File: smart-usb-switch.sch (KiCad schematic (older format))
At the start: 8 parts, among them J1 USB_A, J2 USB_A, J3 Conn_01x04, J4 Conn_01x02, Q1 2N7002E, U1 ESP-12F, U2 TLV75533PDBV

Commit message: more docs, updates
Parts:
- U2: symbol Regulator_Linear:TLV75533PDBV -> smart-usb-switch-rescue:TLV75533PDBV-Regulator_Linear
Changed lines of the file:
@@
 EESchema Schematic File Version 4
-EELAYER 26 0
+EELAYER 30 0
 EELAYER END
 $Descr A4 11693 8268
@@
 	5700 2100 5700 2400
 $Comp
-L Regulator_Linear:TLV75533PDBV U2
+L smart-usb-switch-rescue:TLV75533PDBV-Regulator_Linear U2
 U 1 1 5DE30043
 P 4250 2900

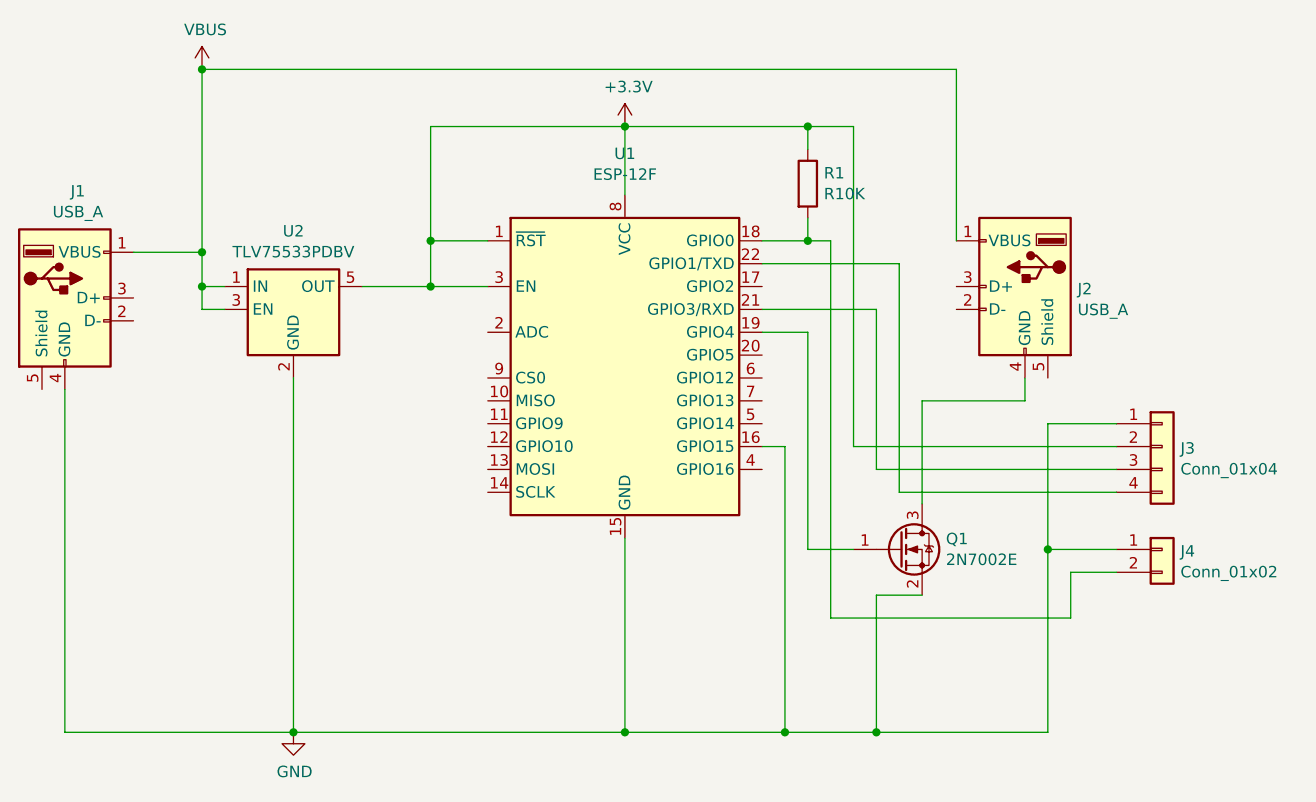
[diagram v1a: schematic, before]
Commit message: reroute
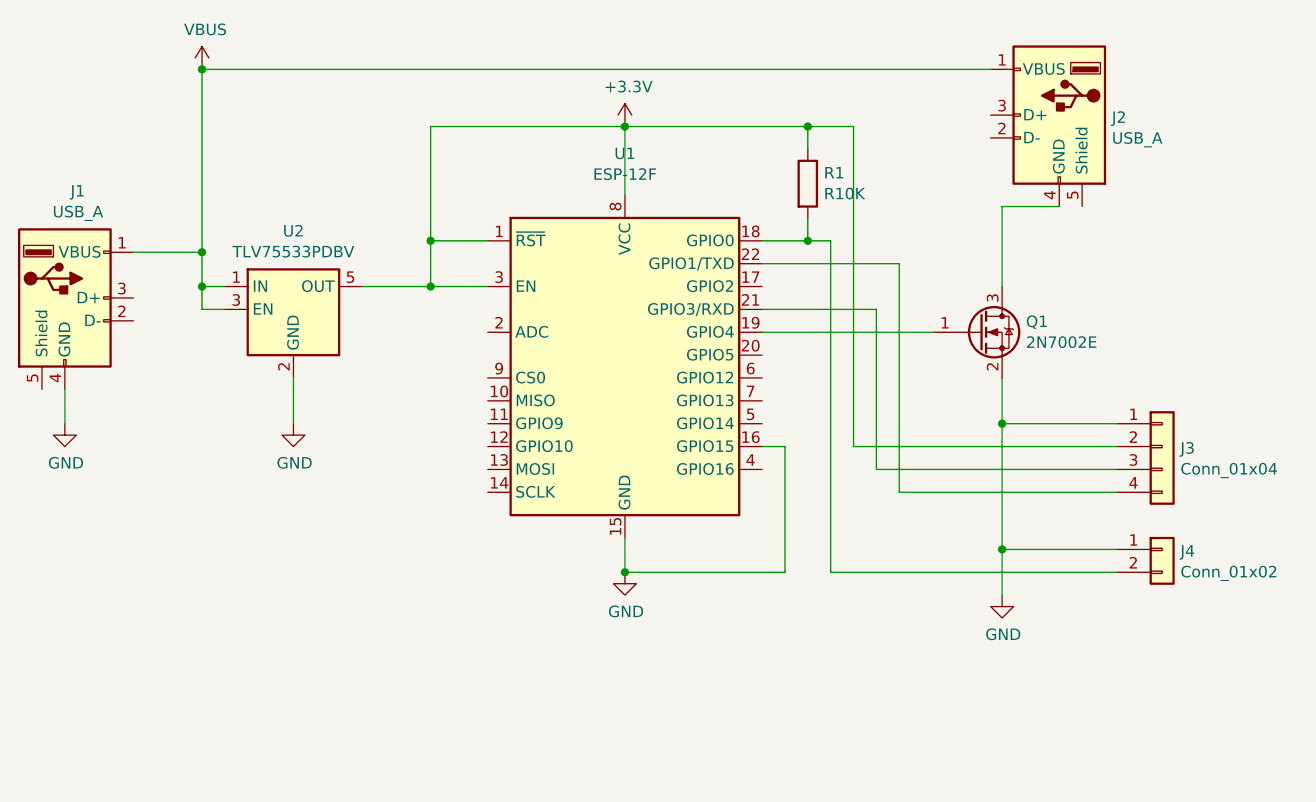
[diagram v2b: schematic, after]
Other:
- moved on the sheet: J2, Q1
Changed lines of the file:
@@
 $EndComp
 Wire Wire Line
-	3250 4750 4250 4750
-Wire Wire Line
-	5700 4750 5700 3900
+	5700 4050 5700 3900
 Wire Wire Line
 	3550 2650 3850 2650
@@
 L Connector:USB_A J2
 U 1 1 5DE34A4B
-P 7450 2800
-F 0 "J2" H 7220 2789 50  0000 R CNN
-F 1 "USB_A" H 7220 2698 50  0000 R CNN
-F 2 "Connector_USB:USB_A_Stewart_SS-52100-001_Horizontal" H 7600 2750 50  0001 C CNN
-F 3 " ~" H 7600 2750 50  0001 C CNN
-	1    7450 2800
+P 7600 2050
+F 0 "J2" H 7370 2039 50  0000 R CNN
+F 1 "USB_A" H 7370 1948 50  0000 R CNN
+F 2 "Connector_USB:USB_A_Stewart_SS-52100-001_Horizontal" H 7750 2000 50  0001 C CNN
+F 3 " ~" H 7750 2000 50  0001 C CNN
+	1    7600 2050
 	-1   0    0    -1
 $EndComp
-Wire Wire Line
-	7450 3200 7450 3300
-Connection ~ 5700 4750
-Wire Wire Line
-	6800 4150 6800 4750
-Connection ~ 6800 4750
-Wire Wire Line
-	6800 4750 6400 4750
-Wire Wire Line
-	6800 4750 7550 4750
+Connection ~ 5700 4050
 $Comp
 L power:GND #PWR0101
 U 1 1 5DE35A33
-P 4250 4750
-F 0 "#PWR0101" H 4250 4500 50  0001 C CNN
-F 1 "GND" H 4255 4577 50  0000 C CNN
-F 2 "" H 4250 4750 50  0001 C CNN
-F 3 "" H 4250 4750 50  0001 C CNN
-	1    4250 4750
+P 4250 3400
+F 0 "#PWR0101" H 4250 3150 50  0001 C CNN
+F 1 "GND" H 4255 3227 50  0000 C CNN
+F 2 "" H 4250 3400 50  0001 C CNN
+F 3 "" H 4250 3400 50  0001 C CNN
+	1    4250 3400
 	1    0    0    -1
 $EndComp
@@
 Connection ~ 5700 2100
 Wire Wire Line
-	7150 2600 7150 1850
-Wire Wire Line
-	7150 1850 3850 1850
-Wire Wire Line
 	3850 1850 3850 2650
 Connection ~ 3850 2650
-Wire Wire Line
-	6800 4150 7000 4150
 $Comp
 L Connector_Generic:Conn_01x04 J3
@@
 	6700 2100 6500 2100
 Wire Wire Line
-	7850 3400 7550 3400
-Wire Wire Line
-	7550 3400 7550 3950
-Wire Wire Line
 	6800 2900 6800 3600
 $Comp
@@
 	6300 2600 6500 2600
 Wire Wire Line
-	6600 2600 6600 4250
-Wire Wire Line
-	7850 4050 7650 4050
-Wire Wire Line
-	6700 3950 6500 3950
-Wire Wire Line
-	6600 4250 7650 4250
-Wire Wire Line
-	7650 4250 7650 4050
-Wire Wire Line
-	7550 3950 7850 3950
-Connection ~ 7550 3950
-Wire Wire Line
-	7550 3950 7550 4750
-Wire Wire Line
-	4250 3200 4250 4750
-Connection ~ 4250 4750
+	6600 2600 6600 4050
+Wire Wire Line
+	7350 3950 7850 3950
+Wire Wire Line
+	4250 3200 4250 3400
 $Comp
 L Transistor_FET:2N7002E Q1
 U 1 1 5DE386B7
-P 6900 3950
-F 0 "Q1" H 7104 3996 50  0000 L CNN
-F 1 "2N7002E" H 7104 3905 50  0000 L CNN
-F 2 "Package_TO_SOT_SMD:SOT-23" H 7100 3875 50  0001 L CIN
-F 3 "http://www.diodes.com/assets/Datasheets/ds30376.pdf" H 6900 3950 50  0001 L CNN
-	1    6900 3950
+P 7250 3000
+F 0 "Q1" H 7454 3046 50  0000 L CNN
+F 1 "2N7002E" H 7454 2955 50  0000 L CNN
+F 2 "Package_TO_SOT_SMD:SOT-23" H 7450 2925 50  0001 L CIN
+F 3 "http://www.diodes.com/assets/Datasheets/ds30376.pdf" H 7250 3000 50  0001 L CNN
+	1    7250 3000
 	1    0    0    -1
 $EndComp
@@
 	6300 3500 6400 3500
 Wire Wire Line
-	6400 3500 6400 4750
-Connection ~ 6400 4750
-Wire Wire Line
-	6400 4750 5700 4750
+	6400 3500 6400 4050
+Wire Wire Line
+	6400 4050 5700 4050
 $Comp
 L Device:R R1
@@
 Connection ~ 3850 1850
 Wire Wire Line
-	4250 4750 5700 4750
-Wire Wire Line
-	3250 3250 3250 4750
-Wire Wire Line
-	7000 3750 7000 3300
-Wire Wire Line
-	7000 3300 7450 3300
-Wire Wire Line
-	6500 3000 6300 3000
-Wire Wire Line
-	6500 3000 6500 3950
+	3250 3250 3250 3400
+Wire Wire Line
+	7350 2800 7350 2450
+Wire Wire Line
+	7350 2450 7600 2450
 Wire Wire Line
 	6700 3500 6700 2100
@@
 Wire Wire Line
 	6900 3700 7850 3700
+$Comp
+L power:GND #PWR?
+U 1 1 5DF189E7
+P 3250 3400
+F 0 "#PWR?" H 3250 3150 50  0001 C CNN
+F 1 "GND" H 3255 3227 50  0000 C CNN
+F 2 "" H 3250 3400 50  0001 C CNN
+F 3 "" H 3250 3400 50  0001 C CNN
+	1    3250 3400
+	1    0    0    -1
+$EndComp
+$Comp
+L power:GND #PWR?
+U 1 1 5DF18E62
+P 5700 4050
+F 0 "#PWR?" H 5700 3800 50  0001 C CNN
+F 1 "GND" H 5705 3877 50  0000 C CNN
+F 2 "" H 5700 4050 50  0001 C CNN
+F 3 "" H 5700 4050 50  0001 C CNN
+	1    5700 4050
+	1    0    0    -1
+$EndComp
+$Comp
+L power:GND #PWR?
+U 1 1 5DF19647
+P 7350 4150
+F 0 "#PWR?" H 7350 3900 50  0001 C CNN
+F 1 "GND" H 7355 3977 50  0000 C CNN
+F 2 "" H 7350 4150 50  0001 C CNN
+F 3 "" H 7350 4150 50  0001 C CNN
+	1    7350 4150
+	1    0    0    -1
+$EndComp
+Wire Wire Line
+	3850 1850 7300 1850
+Wire Wire Line
+	6600 4050 7850 4050
+Wire Wire Line
+	6300 3000 7050 3000
+Wire Wire Line
+	7350 3200 7350 3400
+Connection ~ 7350 3400
+Wire Wire Line
+	7350 3400 7350 3950
+Wire Wire Line
+	7350 3400 7850 3400
+Connection ~ 7350 3950
+Wire Wire Line
+	7350 3950 7350 4150
 $EndSCHEMATC
